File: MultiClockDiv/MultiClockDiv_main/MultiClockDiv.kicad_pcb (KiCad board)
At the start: 2 copper layers, 38.1 x 105 mm, 32 parts, among them J1 GATE OUT1, J2 GATE OUT2, J3 MASTER CLOCK OUT, J4 EXTERNAL CLOCK IN, J5 Conn_01x16_Male, SW1 SW_SPDT

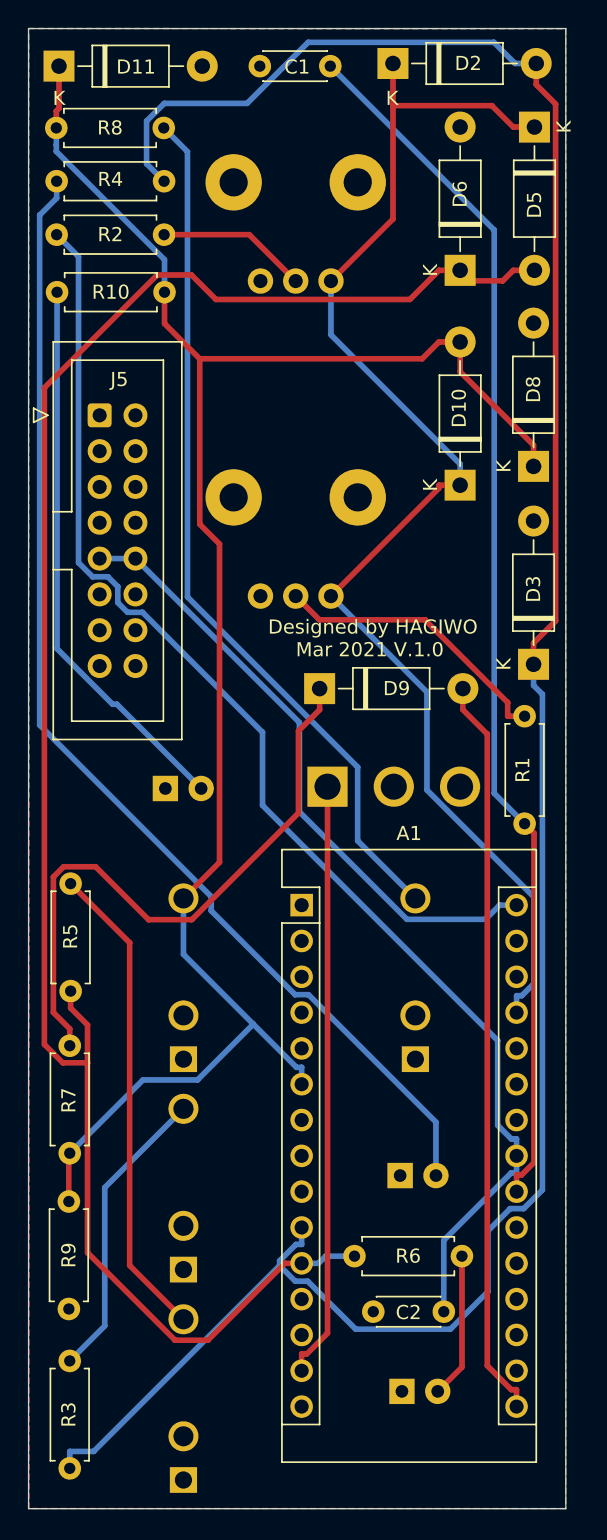
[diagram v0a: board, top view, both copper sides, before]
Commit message: correct
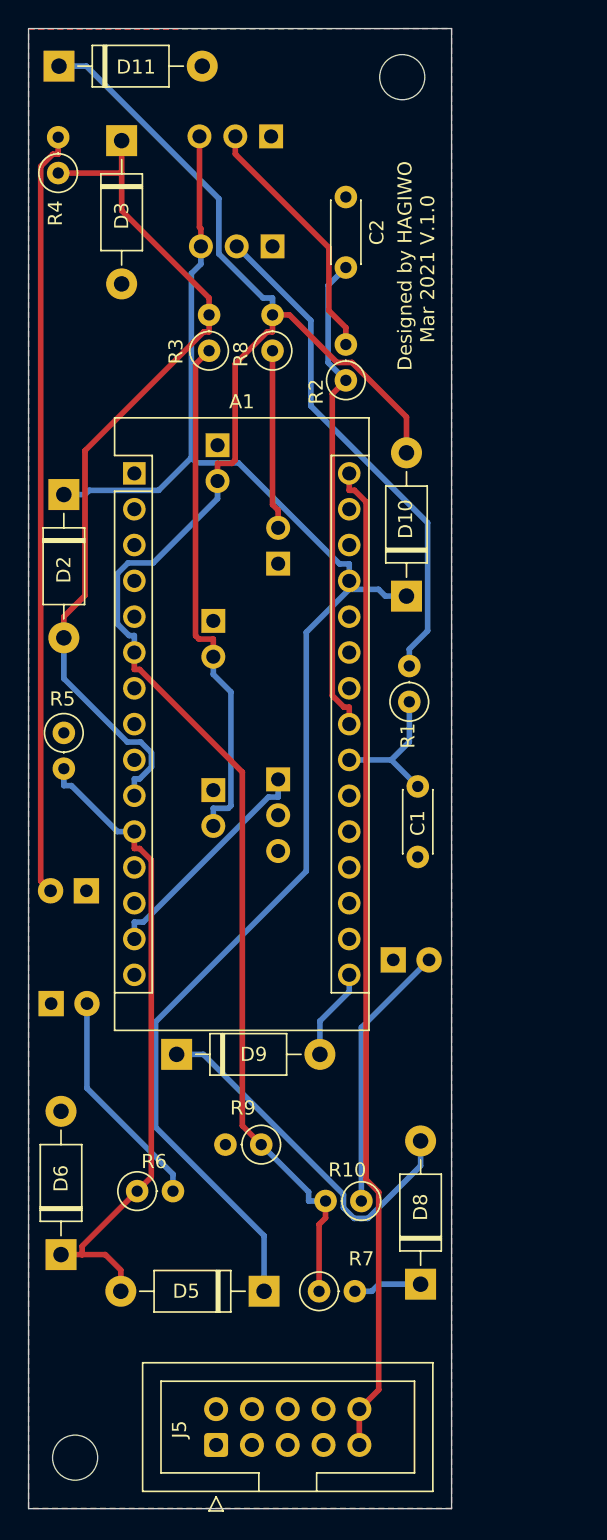
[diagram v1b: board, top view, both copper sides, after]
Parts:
- removed RV1, RV2: 100K, Potentiometer_THT:Potentiometer_Alps_RK09K_Single_Vertical
- added ?: , , F.Cu at (182.8, 92.8)
- added ?: , , F.Cu at (182.1, 84.5)
- added H5: MountingHole, MountingHole:MountingHole_3.2mm_M3, F.Cu at (165.1, 149.1)
- added H6: MountingHole, MountingHole:MountingHole_3.2mm_M3, F.Cu at (188.3, 51.2)
- added MULTI/DIV1: 100K, Connector_PinHeader_2.54mm:PinHeader_1x03_P2.54mm_Vertical, B.Cu at (179.1, 63.2)
- added RATE1: 100K, Connector_PinHeader_2.54mm:PinHeader_1x03_P2.54mm_Vertical, B.Cu at (179.0, 55.4)
- J1, J2, J3, J4: footprint Connector_Audio:Jack_3.5mm_QingPu_WQP-PJ398SM_Vertical_CircularHoles -> Connector_PinHeader_2.54mm:PinHeader_1x02_P2.54mm_Vertical
- J5: value Conn_01x16_Male -> POWER; footprint Connector_IDC:IDC-Header_2x08_P2.54mm_Vertical -> Connector_IDC:IDC-Header_2x05_P2.54mm_Vertical
- R1, R10, R2, R3, R4, R5, R6, R7, R8, R9: footprint Resistor_THT:R_Axial_DIN0207_L6.3mm_D2.5mm_P7.62mm_Horizontal -> Resistor_THT:R_Axial_DIN0207_L6.3mm_D2.5mm_P2.54mm_Vertical
- SW1: value SW_SPDT -> SELECT; footprint digikey-footprints:Toggle_Switch_100SP1T1B4M2QE -> Connector_PinHeader_2.54mm:PinHeader_1x03_P2.54mm_Vertical
- moved D5 84.8 mm to (178.5, 137.3), turned to 180 degrees
- moved C2 79.1 mm to (184.3, 59.7), turned to 270 degrees
- moved D6 75.3 mm to (164.1, 134.7)
- moved J5 73.5 mm to (175.1, 148.2), turned to 90 degrees
- moved R3 72.3 mm to (174.6, 70.6), turned to 90 degrees
- moved R10 68.0 mm to (185.4, 130.9), turned to 180 degrees
- moved D8 58.5 mm to (189.6, 136.8)
- moved C1 51.5 mm to (189.4, 101.5), turned to 270 degrees
- moved J2 49.0 mm to (174.9, 101.8), turned to 180 degrees
- moved D3 47.2 mm to (168.4, 55.7), turned to 270 degrees
- moved J1 46.1 mm to (174.9, 89.8), turned to 180 degrees
- moved J3 43.6 mm to (175.2, 77.3), turned to 180 degrees
- moved D2 38.5 mm to (164.3, 80.8), turned to 270 degrees
- moved D4 37.1 mm to (163.4, 116.9)
- moved J4 36.5 mm to (179.5, 85.7)
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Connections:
- net 12V renamed Net-(A1-Pad30)
- A1 pad 1: Net-(A1-Pad1) -> (no net)
- A1 pad 12: Net-(A1-Pad12) -> (no net)
- A1 pad 13: Net-(A1-Pad13) -> (no net)
- A1 pad 15: Net-(A1-Pad15) -> (no net)
- A1 pad 17: Net-(A1-Pad17) -> (no net)
- A1 pad 18: Net-(A1-Pad18) -> (no net)
- A1 pad 19: Net-(A1-Pad19) -> (no net)
- A1 pad 2: Net-(A1-Pad2) -> (no net)
- A1 pad 20: Net-(A1-Pad20) -> (no net)
- A1 pad 21: Net-(A1-Pad21) -> (no net)
- A1 pad 24: Net-(A1-Pad24) -> (no net)
- A1 pad 25: Net-(A1-Pad25) -> (no net)
- A1 pad 26: Net-(A1-Pad26) -> (no net)
- A1 pad 28: Net-(A1-Pad28) -> (no net)
- A1 pad 29: Net-(A1-Pad29) -> (no net)
- A1 pad 3: Net-(A1-Pad3) -> (no net)
- A1 pad 5: Net-(A1-Pad5) -> (no net)
- A1 pad 7: Net-(A1-Pad7) -> (no net)
- A1 pad 8: Net-(A1-Pad8) -> (no net)
- A1 pad 9: Net-(A1-Pad9) -> (no net)
- D8 pad 1: Net-(A1-Pad6) -> Net-(D8-Pad1)
- D8 pad 2: GND -> Net-(D8-Pad2)
- D9 pad 1: Net-(D9-Pad1) -> Net-(D8-Pad2)
- J5 pad 1: Net-(J5-Pad1) -> (no net)
- J5 pad 2: Net-(J5-Pad2) -> (no net)
- R7 pad 2: Net-(D9-Pad1) -> Net-(D8-Pad1)
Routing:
- net Net-(A1-Pad10): track 169.0 -> 61.9 mm
- net Net-(A1-Pad11): track 133.9 -> 46.5 mm
- net Net-(A1-Pad22): track 86.5 -> 10.3 mm
- net Net-(A1-Pad23): track 93.7 -> 34.5 mm
- net Net-(J4-PadT): track 62.0 -> 12.7 mm
- net Net-(A1-Pad16): track 52.7 -> 6.50 mm
- net Net-(D9-Pad1): track 44.3 -> 0.00 mm
- net Net-(J2-PadT): track 34.2 -> 0.00 mm
- net Net-(D1-Pad2): track 83.2 -> 54.5 mm
- net Net-(A1-Pad30): track 44.3 -> 70.6 mm
- net Net-(A1-Pad14): track 42.4 -> 16.3 mm
- net Net-(D8-Pad2): track 0.00 -> 26.0 mm
- net Net-(D7-Pad2): track 39.6 -> 19.1 mm
- net 5V: track 95.0 -> 112.3 mm
- net Net-(J1-PadT): track 21.2 -> 36.9 mm
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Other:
- board size 38.1 x 105 mm -> 30 x 105 mm
- board text added: "1"
- board text added: "3"
- board text added: "CLOCK IN"
- board text added: "CLOCK OUT"
- board text added: "GATE OUT1"
- board text added: "GATE OUT2"
- board text added: "SELECT SW"
